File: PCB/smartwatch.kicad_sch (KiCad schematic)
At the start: 24 parts, among them J1 Serial wire/Charging, J2 Battery input, SW1 SW_Push, U1 STM32L432KBUx, U2 LSM6DS3, U3 W25Q128JVPIQ, U4 TP4056, U5 LT1761-3.3, X2 20Mhz, Y2 LSE 32khz

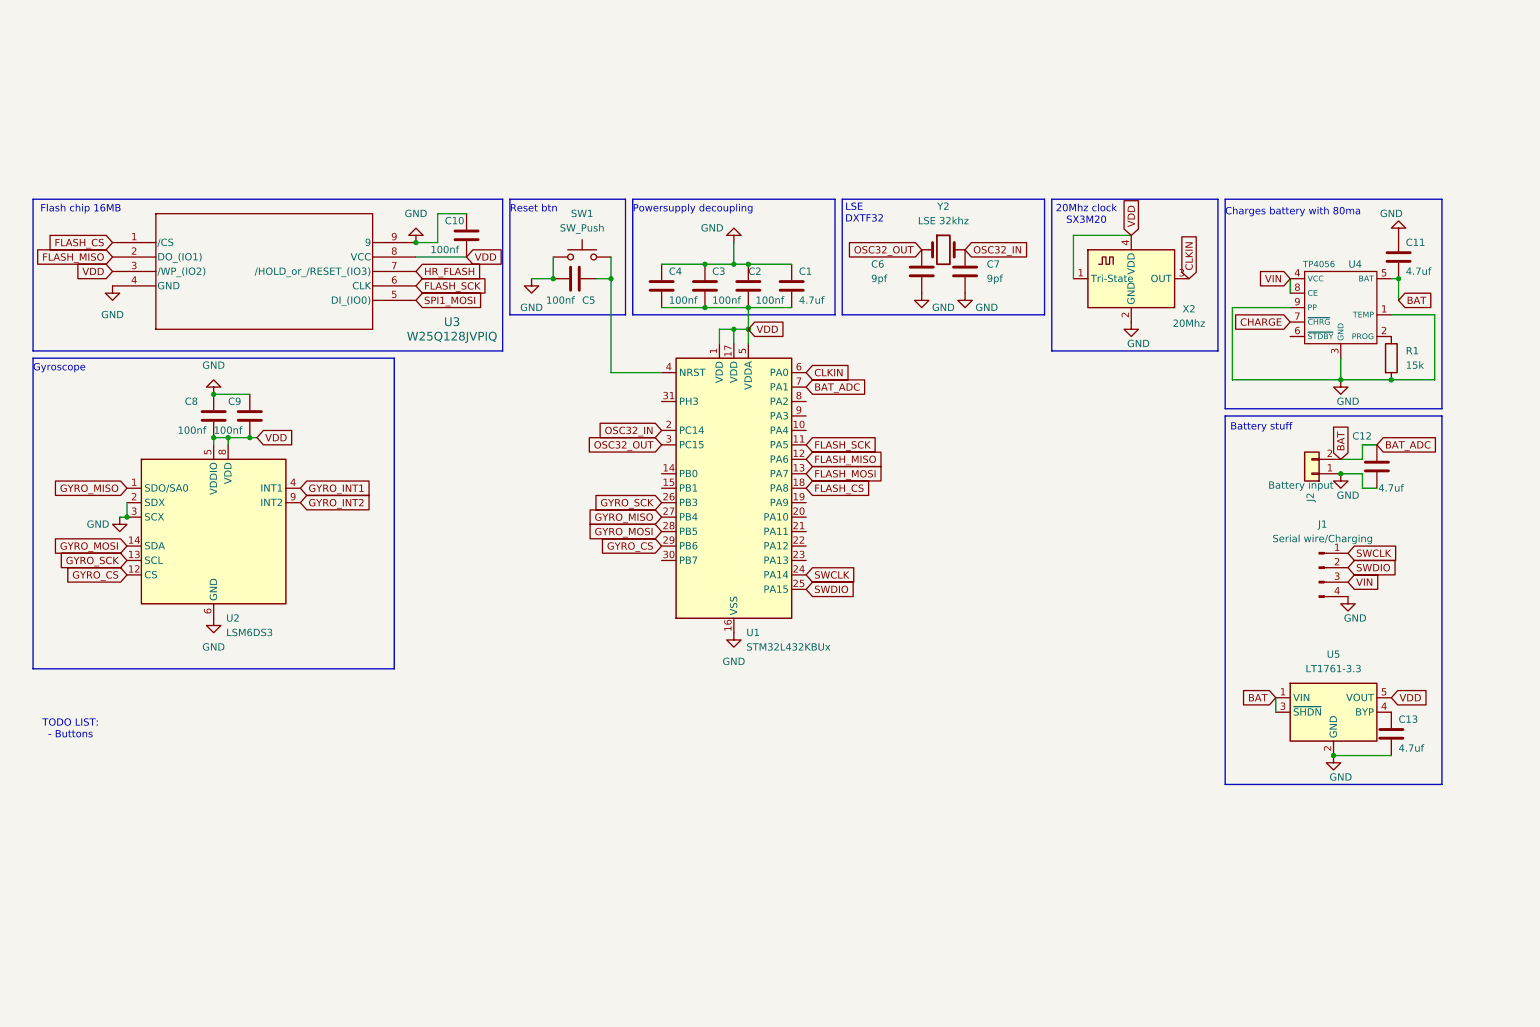
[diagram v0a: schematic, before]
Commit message: All but routing done
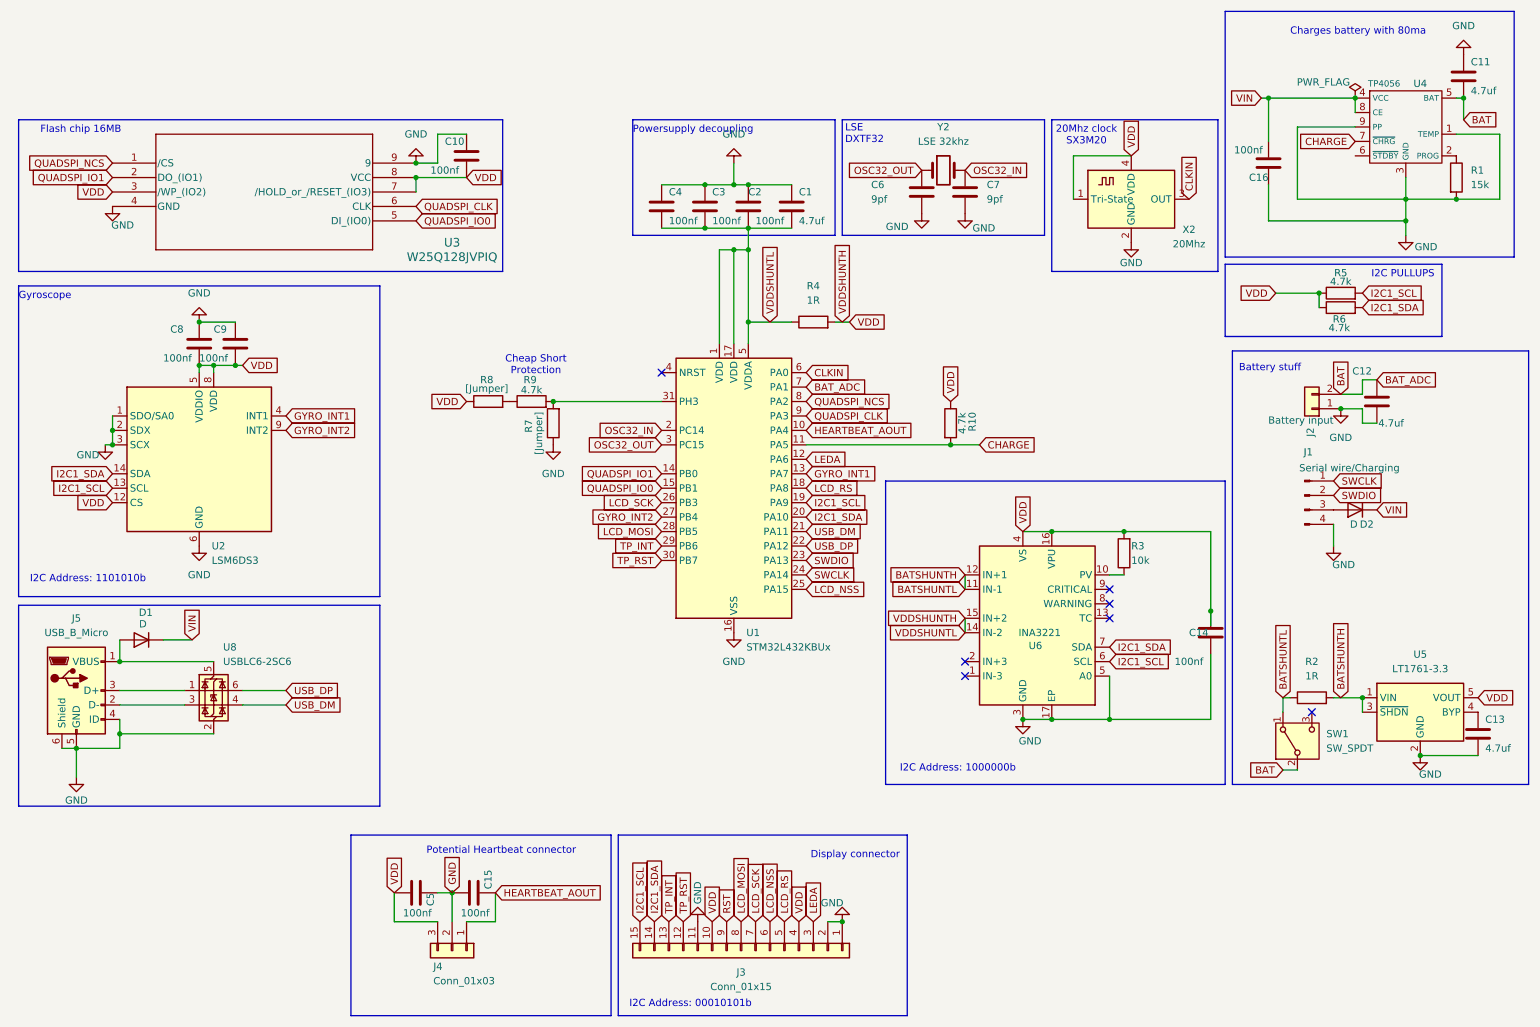
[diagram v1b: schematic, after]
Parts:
- removed SW1: SW_Push, symbol Switch:SW_Push
- added C14, C15, C16: 100nf, Capacitor_SMD:C_0603_1608Metric, symbol Device:C
- added D1, D2: D, Diode_SMD:D_0201_0603Metric, symbol Device:D
- added J3: Conn_01x15, Connector_FFC-FPC:TE_1-1734839-5_1x15-1MP_P0.5mm_Horizontal, symbol Connector_Generic:Conn_01x15
- added J4: Conn_01x03, Connector_FFC-FPC:TE_0-1734839-5_1x05-1MP_P0.5mm_Horizontal, symbol Connector_Generic:Conn_01x03
- added J5: USB_B_Micro, Connector_USB:USB_Micro-B_Amphenol_10118194_Horizontal, symbol Connector:USB_B_Micro
- added R10, R5, R6, R9: 4.7k, Resistor_SMD:R_0805_2012Metric, symbol Device:R
- added R2, R4: 1R, Resistor_SMD:R_0805_2012Metric, symbol Device:R
- added R3: 10k, Resistor_SMD:R_0805_2012Metric, symbol Device:R
- added R7, R8: [Jumper], Resistor_SMD:R_0805_2012Metric, symbol Device:R
- added SW1: SW_SPDT, MyButtons:MSK12CO2, symbol Switch:SW_SPDT
- added U6: INA3221, Package_DFN_QFN:Texas_RGV0016A_VQFN-16-1EP_4x4mm_P0.65mm_EP2.1x2.1mm, symbol Power_Management:INA3221
- added U8: USBLC6-2SC6, Package_TO_SOT_SMD:SOT-23-6, symbol Power_Protection:USBLC6-2SC6
- J1: footprint Connector_PinHeader_2.54mm:PinHeader_1x04_P2.54mm_Horizontal -> Connector_PinHeader_2.54mm:PinHeader_1x04_P2.54mm_Vertical
- J2: footprint (none) -> Connector_PinHeader_2.54mm:PinHeader_1x02_P2.54mm_Vertical
- R1: footprint (none) -> Resistor_SMD:R_0805_2012Metric
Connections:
- net FLASH_MOSI is gone; now on net GYRO_INT1: U1.13 (PA7)
- net HR_FLASH is gone; now on net VDD: U3.7 (/HOLD_or_/RESET_(IO3))
- net SPI1_MOSI is gone; now on net QUADSPI_IO0: U3.5 (DI_(IO0))
- net BAT: now also SW1.2 (B); no longer U5.1 (VIN), U5.3 (~{SHDN})
- net CHARGE: now also U1.11 (PA5), R10.2
- net GND: now also C5.1, U2.1 (SDO/SA0), C14.2, C15.2, C16.1, J3.1 (Pin_1), J3.11 (Pin_11), J3.2 (Pin_2), J4.2 (Pin_2), J5.4 (ID), J5.5 (GND), J5.6 (Shield), R7.1, U6.17 (EP), U6.3 (GND), U6.5 (A0), U8.2 (GND); no longer C5.2
- net GYRO_INT2: now also U1.27 (PB4)
- net SWDIO: now also U1.23 (PA13); no longer U1.25 (PA15)
- net VDD: now also C5.2, U2.12 (CS), C14.1, J3.10 (Pin_10), J3.4 (Pin_4), J4.3 (Pin_3), R10.1, R3.2, R4.1, R4.2, R5.1, R6.1, R8.1, U6.14 (IN-2), U6.15 (IN+2), U6.16 (VPU), U6.4 (VS)
- net VIN: now also C16.2, D1.1 (K), D2.1 (K); no longer J1.3 (Pin_3)
- net at U1.4 (NRST): no longer C5.1
- net HEARTBEAT_AOUT: now reaches U1.10 (PA4)
- net HEARTBEAT_AOUT: now also C15.1, J4.1 (Pin_1)
- net QUADSPI_IO1: now reaches U1.14 (PB0)
- net QUADSPI_IO1: now also U3.2 (DO_(IO1))
- net QUADSPI_IO0: now reaches U1.15 (PB1)
- net I2C1_SCL: now reaches U1.19 (PA9)
- net I2C1_SCL: now also U2.13 (SCL), J3.15 (Pin_15), R5.2, U6.6 (SCL)
- net I2C1_SDA: now reaches U1.20 (PA10)
- net I2C1_SDA: now also U2.14 (SDA), J3.14 (Pin_14), R6.2, U6.7 (SDA)
- net USB_DM: now reaches U1.21 (PA11)
- net USB_DM: now also U8.4 (I/O2)
- net USB_DP: now reaches U1.22 (PA12)
- net USB_DP: now also U8.6 (I/O1)
- net TP_RST: now reaches U1.30 (PB7)
- net TP_RST: now also J3.12 (Pin_12)
- net at U1.31 (PH3): now also R7.2, R9.2
- net QUADSPI_NCS: now reaches U1.8 (PA2)
- net QUADSPI_NCS: now also U3.1 (/CS)
- net QUADSPI_CLK: now reaches U1.9 (PA3)
- net QUADSPI_CLK: now also U3.6 (CLK)
- net FLASH_CS renamed LCD_RS
- net LCD_RS: now also J3.5 (Pin_5); no longer U3.1 (/CS)
- net FLASH_MISO renamed LEDA
- net LEDA: now also J3.3 (Pin_3); no longer U3.2 (DO_(IO1))
- removed net FLASH_SCK: U1.11 (PA5), U3.6 (CLK)
- net GYRO_CS renamed TP_INT
- net TP_INT: now also J3.13 (Pin_13); no longer U2.12 (CS)
- removed net GYRO_MISO: U1.27 (PB4), U2.1 (SDO/SA0)
- net GYRO_MOSI renamed LCD_MOSI
- net LCD_MOSI: now also J3.8 (Pin_8); no longer U2.14 (SDA)
- net GYRO_SCK renamed LCD_SCK
- net LCD_SCK: now also J3.7 (Pin_7); no longer U2.13 (SCL)
- new net: D2.2 (A), J1.3 (Pin_3)
- new net: R8.2, R9.1
- new net: D1.2 (A), J5.1 (VBUS), U8.5 (VBUS)
- new net: J5.3 (D+), U8.1 (I/O1)
- new net: J5.2 (D-), U8.3 (I/O2)
- new net: R3.1, U6.10 (PV)
- new net BATSHUNTH: R2.1, R2.2, SW1.1 (A), U5.1 (VIN), U5.3 (~{SHDN}), U6.11 (IN-1), U6.12 (IN+1)
- new net LCD_NSS: J3.6 (Pin_6), U1.25 (PA15)
- new net RST: J3.9 (Pin_9)
- no-connect marks 0 -> 7
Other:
- note added: "Cheap Short Protection"
- note added: "Display connector"
- note added: "I2C Address: 00010101b"
- note added: "I2C Address: 1000000b"
- note added: "I2C Address: 1101010b"
- note added: "I2C PULLUPS"
- note added: "Potential Heartbeat connector"
- note removed: "Reset btn"
- note removed: "TODO LIST: - Buttons"
- moved on the sheet: C1, C10, C11, C12, C13, C2, C3, C4, C6, C7, C8, C9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
